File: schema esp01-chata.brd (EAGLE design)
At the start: 44.1 x 35.5 mm, 10 parts

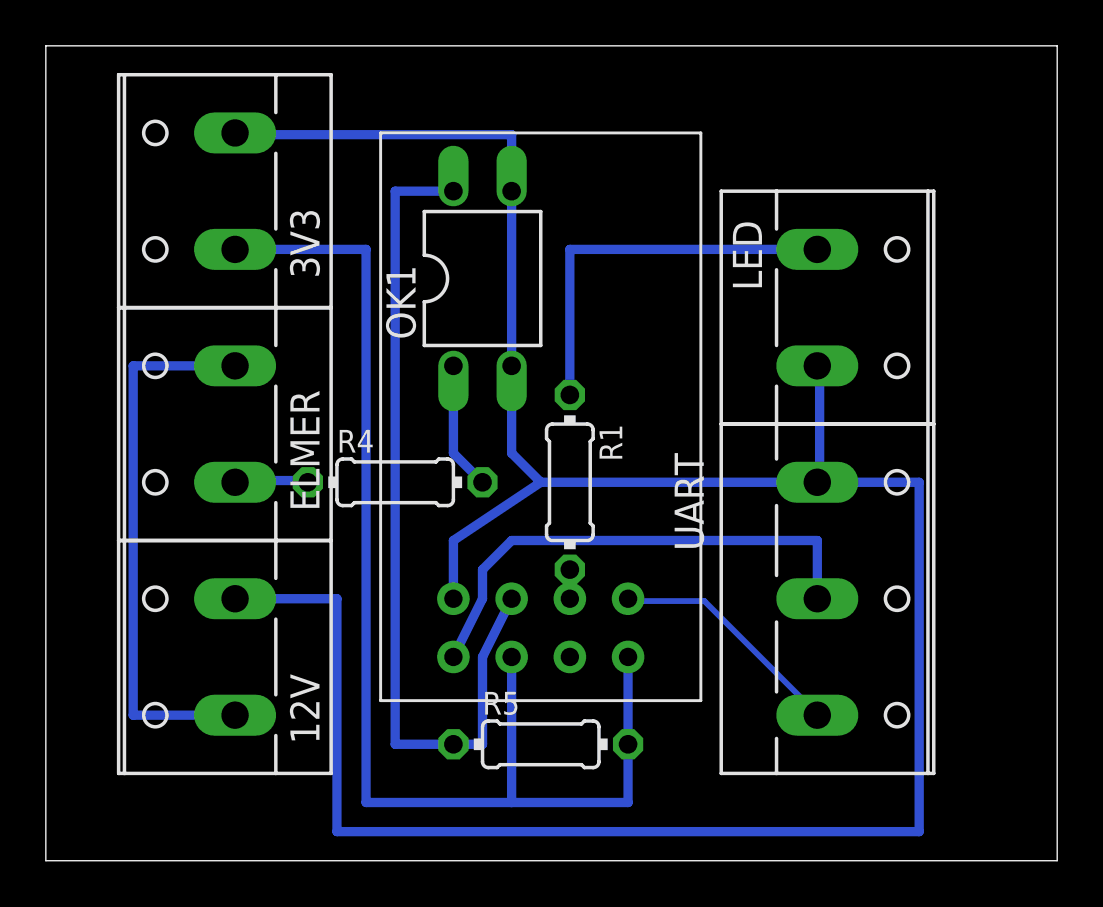
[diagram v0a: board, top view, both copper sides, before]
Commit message: zmeny eagle
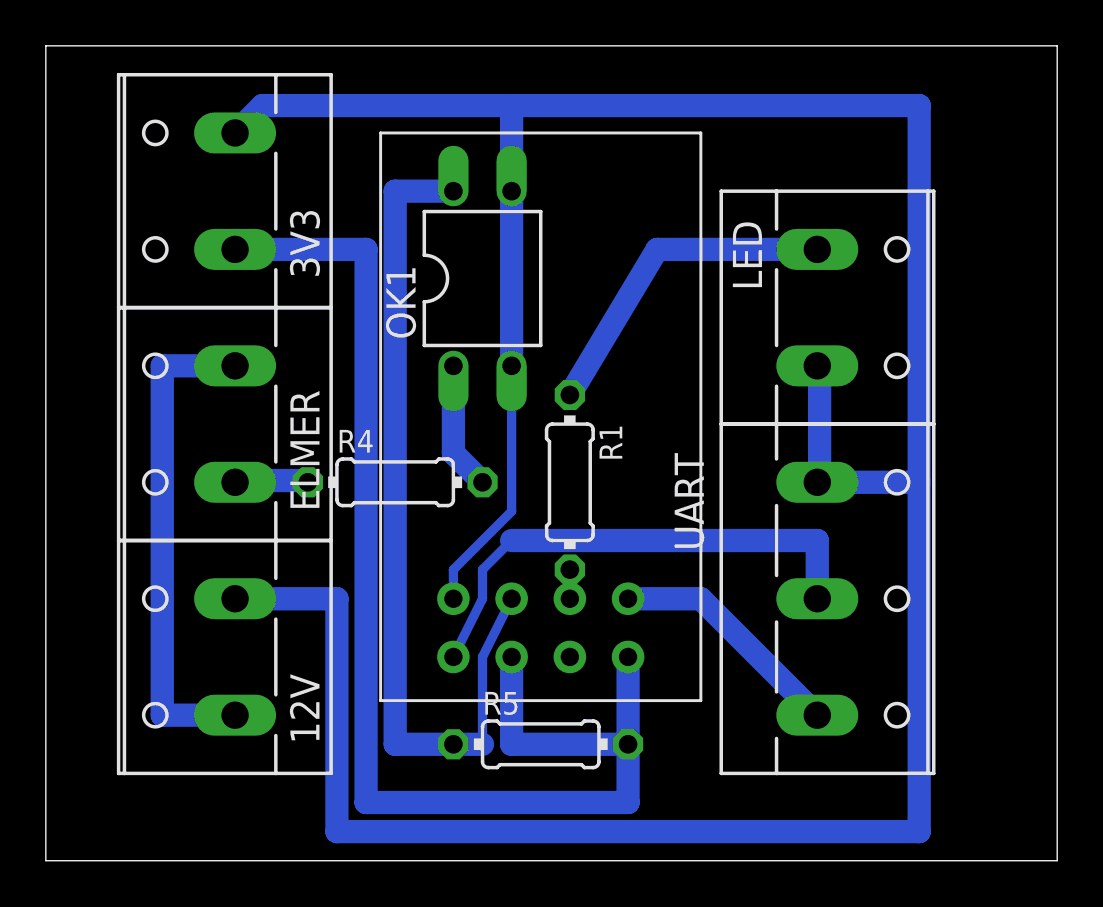
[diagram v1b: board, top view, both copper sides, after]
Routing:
- net GND: track 112.4 -> 134.3 mm
- net N$2: track 17.1 -> 14.4 mm
- net +12V: track 24.1 -> 21.6 mm
- net +3V3: track 54.0 -> 56.5 mm
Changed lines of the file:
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@@
 <?xml version="1.0" encoding="utf-8"?>
 <!DOCTYPE eagle SYSTEM "eagle.dtd">
-<eagle version="7.3.0">
+<eagle version="6.5.0">
 <drawing>
 <settings>
@@
 <pass name="Default">
 <param name="RoutingGrid" value="50mil"/>
-<param name="AutoGrid" value="1"/>
-<param name="Efforts" value="0"/>
-<param name="TopRouterVariant" value="1"/>
 <param name="tpViaShape" value="round"/>
 <param name="PrefDir.1" value="0"/>
@@
 <contactref element="LED" pad="1"/>
 <contactref element="R1" pad="1"/>
-<wire x1="29.845" y1="26.67" x2="19.05" y2="26.67" width="0.4064" layer="16"/>
-<wire x1="19.05" y1="26.67" x2="19.05" y2="20.32" width="0.4064" layer="16"/>
+<wire x1="29.845" y1="26.67" x2="22.86" y2="26.67" width="1.016" layer="16"/>
+<wire x1="22.86" y1="26.67" x2="19.05" y2="20.32" width="1.016" layer="16"/>
 </signal>
 <signal name="N$3">
 <contactref element="R1" pad="2"/>
 <contactref element="U$1" pad="P$6"/>
-<wire x1="19.2024" y1="11.557" x2="19.2024" y2="12.7" width="0.254" layer="16"/>
-<wire x1="19.2024" y1="12.7" x2="19.05" y2="12.7" width="0.254" layer="16"/>
-<wire x1="19.2024" y1="11.557" x2="19.05" y2="11.43" width="0.254" layer="16"/>
+<wire x1="19.05" y1="12.7" x2="19.05" y2="11.43" width="0.4064" layer="16"/>
 </signal>
 <signal name="+3V3">
+<contactref element="R5" pad="2"/>
+<wire x1="10.16" y1="26.67" x2="10.16" y2="2.54" width="1.016" layer="16"/>
+<wire x1="10.16" y1="2.54" x2="21.59" y2="2.54" width="1.016" layer="16"/>
+<wire x1="21.59" y1="2.54" x2="21.59" y2="5.08" width="1.016" layer="16"/>
 <contactref element="3V3" pad="1"/>
 <contactref element="U$1" pad="P$4"/>
+<wire x1="21.59" y1="5.08" x2="21.59" y2="8.89" width="1.016" layer="16"/>
+<wire x1="16.51" y1="5.08" x2="21.59" y2="5.08" width="1.016" layer="16"/>
 <contactref element="U$1" pad="P$2"/>
-<contactref element="R5" pad="2"/>
-<wire x1="4.445" y1="26.67" x2="10.16" y2="26.67" width="0.4064" layer="16"/>
-<wire x1="10.16" y1="26.67" x2="10.16" y2="2.54" width="0.4064" layer="16"/>
-<wire x1="10.16" y1="2.54" x2="16.51" y2="2.54" width="0.4064" layer="16"/>
-<wire x1="16.51" y1="2.54" x2="21.59" y2="2.54" width="0.4064" layer="16"/>
-<wire x1="21.59" y1="2.54" x2="21.59" y2="5.08" width="0.4064" layer="16"/>
-<wire x1="21.59" y1="5.08" x2="21.59" y2="8.89" width="0.4064" layer="16"/>
-<wire x1="16.51" y1="8.89" x2="16.51" y2="2.54" width="0.4064" layer="16"/>
+<wire x1="4.445" y1="26.67" x2="10.16" y2="26.67" width="1.016" layer="16"/>
+<wire x1="16.51" y1="5.08" x2="16.51" y2="8.89" width="1.016" layer="16"/>
 </signal>
 <signal name="N$5">
 <contactref element="U$1" pad="P$5"/>
 <contactref element="UART" pad="3"/>
-<wire x1="24.9174" y1="11.3284" x2="21.717" y2="11.3284" width="0.254" layer="16"/>
-<wire x1="29.718" y1="6.5278" x2="24.9174" y2="11.3284" width="0.254" layer="16"/>
-<wire x1="21.717" y1="11.3284" x2="21.59" y2="11.43" width="0.254" layer="16"/>
-<wire x1="29.718" y1="6.5278" x2="29.845" y2="6.35" width="0.254" layer="16"/>
+<wire x1="21.59" y1="11.43" x2="24.765" y2="11.43" width="1.016" layer="16"/>
+<wire x1="24.765" y1="11.43" x2="29.845" y2="6.35" width="1.016" layer="16"/>
 </signal>
 <signal name="N$6">
 <contactref element="U$1" pad="P$1"/>
 <contactref element="UART" pad="2"/>
-<wire x1="29.845" y1="11.43" x2="29.845" y2="13.97" width="0.4064" layer="16"/>
-<wire x1="29.845" y1="13.97" x2="16.51" y2="13.97" width="0.4064" layer="16"/>
+<wire x1="29.845" y1="11.43" x2="29.845" y2="13.97" width="1.016" layer="16"/>
+<wire x1="29.845" y1="13.97" x2="16.51" y2="13.97" width="1.016" layer="16"/>
 <wire x1="16.51" y1="13.97" x2="15.24" y2="12.7" width="0.4064" layer="16"/>
 <wire x1="15.24" y1="12.7" x2="15.24" y2="11.43" width="0.4064" layer="16"/>
@@
 </signal>
 <signal name="N$7">
-<contactref element="OK1" pad="4"/>
 <contactref element="R5" pad="1"/>
 <contactref element="U$1" pad="P$7"/>
-<wire x1="13.97" y1="5.08" x2="11.43" y2="5.08" width="0.4064" layer="16"/>
-<wire x1="11.43" y1="5.08" x2="11.43" y2="29.21" width="0.4064" layer="16"/>
-<wire x1="11.43" y1="29.21" x2="13.97" y2="29.21" width="0.4064" layer="16"/>
+<wire x1="13.97" y1="5.08" x2="11.43" y2="5.08" width="1.016" layer="16"/>
+<wire x1="11.43" y1="5.08" x2="11.43" y2="29.21" width="1.016" layer="16"/>
 <wire x1="16.51" y1="11.43" x2="15.24" y2="8.89" width="0.4064" layer="16"/>
 <wire x1="15.24" y1="8.89" x2="15.24" y2="5.08" width="0.4064" layer="16"/>
-<wire x1="15.24" y1="5.08" x2="13.97" y2="5.08" width="0.4064" layer="16"/>
+<wire x1="15.24" y1="5.08" x2="13.97" y2="5.08" width="1.016" layer="16"/>
+<contactref element="OK1" pad="4"/>
+<wire x1="11.43" y1="29.21" x2="13.97" y2="29.21" width="1.016" layer="16"/>
 </signal>
 <signal name="+12V">
 <contactref element="ELMER" pad="2"/>
 <contactref element="12V" pad="1"/>
-<wire x1="4.445" y1="21.59" x2="0" y2="21.59" width="0.4064" layer="16"/>
-<wire x1="0" y1="21.59" x2="0" y2="6.35" width="0.4064" layer="16"/>
-<wire x1="0" y1="6.35" x2="4.445" y2="6.35" width="0.4064" layer="16"/>
+<wire x1="4.445" y1="21.59" x2="1.27" y2="21.59" width="1.016" layer="16"/>
+<wire x1="1.27" y1="21.59" x2="1.27" y2="6.35" width="1.016" layer="16"/>
+<wire x1="1.27" y1="6.35" x2="4.445" y2="6.35" width="1.016" layer="16"/>
 </signal>
 <signal name="GND">
+<contactref element="3V3" pad="2"/>
+<contactref element="12V" pad="2"/>
 <contactref element="U$1" pad="P$8"/>
 <contactref element="UART" pad="1"/>
+<wire x1="8.89" y1="1.27" x2="34.29" y2="1.27" width="1.016" layer="16"/>
+<wire x1="34.29" y1="1.27" x2="34.29" y2="16.51" width="1.016" layer="16"/>
+<wire x1="34.29" y1="16.51" x2="29.845" y2="16.51" width="1.016" layer="16"/>
+<contactref element="LED" pad="2"/>
+<wire x1="29.9466" y1="21.3868" x2="29.845" y2="21.59" width="0.254" layer="16"/>
+<wire x1="29.9466" y1="16.5862" x2="29.9466" y2="21.4884" width="1.016" layer="16"/>
+<wire x1="29.9466" y1="21.4884" x2="29.845" y2="21.59" width="0.4064" layer="16"/>
 <contactref element="OK1" pad="2"/>
 <contactref element="OK1" pad="3"/>
-<contactref element="12V" pad="2"/>
-<contactref element="3V3" pad="2"/>
-<contactref element="LED" pad="2"/>
-<wire x1="29.9466" y1="16.5862" x2="29.845" y2="16.51" width="0.254" layer="16"/>
-<wire x1="29.9466" y1="21.3868" x2="29.845" y2="21.59" width="0.254" layer="16"/>
-<wire x1="16.4592" y1="21.3868" x2="16.51" y2="21.59" width="0.254" layer="16"/>
-<wire x1="4.572" y1="31.6738" x2="4.445" y2="31.75" width="0.254" layer="16"/>
-<wire x1="16.6878" y1="29.3878" x2="16.51" y2="29.21" width="0.254" layer="16"/>
-<wire x1="4.572" y1="31.6738" x2="16.51" y2="31.6738" width="0.4064" layer="16"/>
-<wire x1="16.51" y1="31.6738" x2="16.51" y2="29.21" width="0.4064" layer="16"/>
-<wire x1="16.51" y1="29.21" x2="16.51" y2="21.59" width="0.4064" layer="16"/>
-<wire x1="16.4592" y1="21.3868" x2="16.51" y2="21.3868" width="0.4064" layer="16"/>
-<wire x1="16.51" y1="21.3868" x2="16.51" y2="17.78" width="0.4064" layer="16"/>
-<wire x1="16.51" y1="17.78" x2="17.78" y2="16.51" width="0.4064" layer="16"/>
-<wire x1="17.78" y1="16.51" x2="29.845" y2="16.51" width="0.4064" layer="16"/>
-<wire x1="29.9466" y1="16.5862" x2="29.9466" y2="21.4884" width="0.4064" layer="16"/>
-<wire x1="29.9466" y1="21.4884" x2="29.845" y2="21.59" width="0.4064" layer="16"/>
-<wire x1="4.445" y1="11.43" x2="8.89" y2="11.43" width="0.4064" layer="16"/>
-<wire x1="8.89" y1="11.43" x2="8.89" y2="1.27" width="0.4064" layer="16"/>
-<wire x1="8.89" y1="1.27" x2="34.29" y2="1.27" width="0.4064" layer="16"/>
-<wire x1="34.29" y1="1.27" x2="34.29" y2="16.51" width="0.4064" layer="16"/>
-<wire x1="34.29" y1="16.51" x2="29.845" y2="16.51" width="0.4064" layer="16"/>
-<wire x1="13.97" y1="11.43" x2="13.97" y2="13.97" width="0.4064" layer="16"/>
-<wire x1="13.97" y1="13.97" x2="17.78" y2="16.51" width="0.4064" layer="16"/>
+<wire x1="16.51" y1="32.9438" x2="16.51" y2="29.21" width="1.016" layer="16"/>
+<wire x1="16.51" y1="29.21" x2="16.51" y2="21.59" width="1.016" layer="16"/>
+<wire x1="4.445" y1="11.43" x2="8.89" y2="11.43" width="1.016" layer="16"/>
+<wire x1="8.89" y1="11.43" x2="8.89" y2="1.27" width="1.016" layer="16"/>
+<wire x1="16.51" y1="21.59" x2="16.51" y2="15.24" width="0.4064" layer="16"/>
+<wire x1="16.51" y1="15.24" x2="13.97" y2="12.7" width="0.4064" layer="16"/>
+<wire x1="13.97" y1="12.7" x2="13.97" y2="11.43" width="0.4064" layer="16"/>
+<wire x1="16.51" y1="32.9438" x2="34.29" y2="32.9438" width="1.016" layer="16"/>
+<wire x1="34.29" y1="32.9438" x2="34.29" y2="16.51" width="1.016" layer="16"/>
+<wire x1="16.51" y1="32.9438" x2="5.6388" y2="32.9438" width="1.016" layer="16"/>
+<wire x1="5.6388" y1="32.9438" x2="4.445" y2="31.75" width="1.016" layer="16"/>
+<wire x1="29.845" y1="16.51" x2="29.9466" y2="16.5862" width="0" layer="19" extent="16-16"/>
 </signal>
 <signal name="N$4">
 <contactref element="OK1" pad="1"/>
 <contactref element="R4" pad="2"/>
-<wire x1="13.97" y1="21.59" x2="13.97" y2="17.78" width="0.4064" layer="16"/>
-<wire x1="13.97" y1="17.78" x2="15.24" y2="16.51" width="0.4064" layer="16"/>
+<wire x1="13.97" y1="21.59" x2="13.97" y2="17.78" width="1.016" layer="16"/>
+<wire x1="13.97" y1="17.78" x2="15.24" y2="16.51" width="1.016" layer="16"/>
 </signal>
 <signal name="N$8">
@@
 <wire x1="7.5438" y1="16.5862" x2="7.62" y2="16.51" width="0.254" layer="16"/>
 <wire x1="4.572" y1="16.5862" x2="4.445" y2="16.51" width="0.254" layer="16"/>
-<wire x1="7.5438" y1="16.5862" x2="4.445" y2="16.5862" width="0.4064" layer="16"/>
+<wire x1="7.5438" y1="16.5862" x2="4.445" y2="16.5862" width="1.016" layer="16"/>
 <wire x1="4.445" y1="16.5862" x2="4.445" y2="16.51" width="0.4064" layer="16"/>
 </signal>
